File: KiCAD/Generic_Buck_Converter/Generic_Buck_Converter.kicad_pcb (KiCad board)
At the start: 4 copper layers, 17.8 x 25 mm, 20 parts, among them IC1 MAX17634C, J1 Conn_01x03

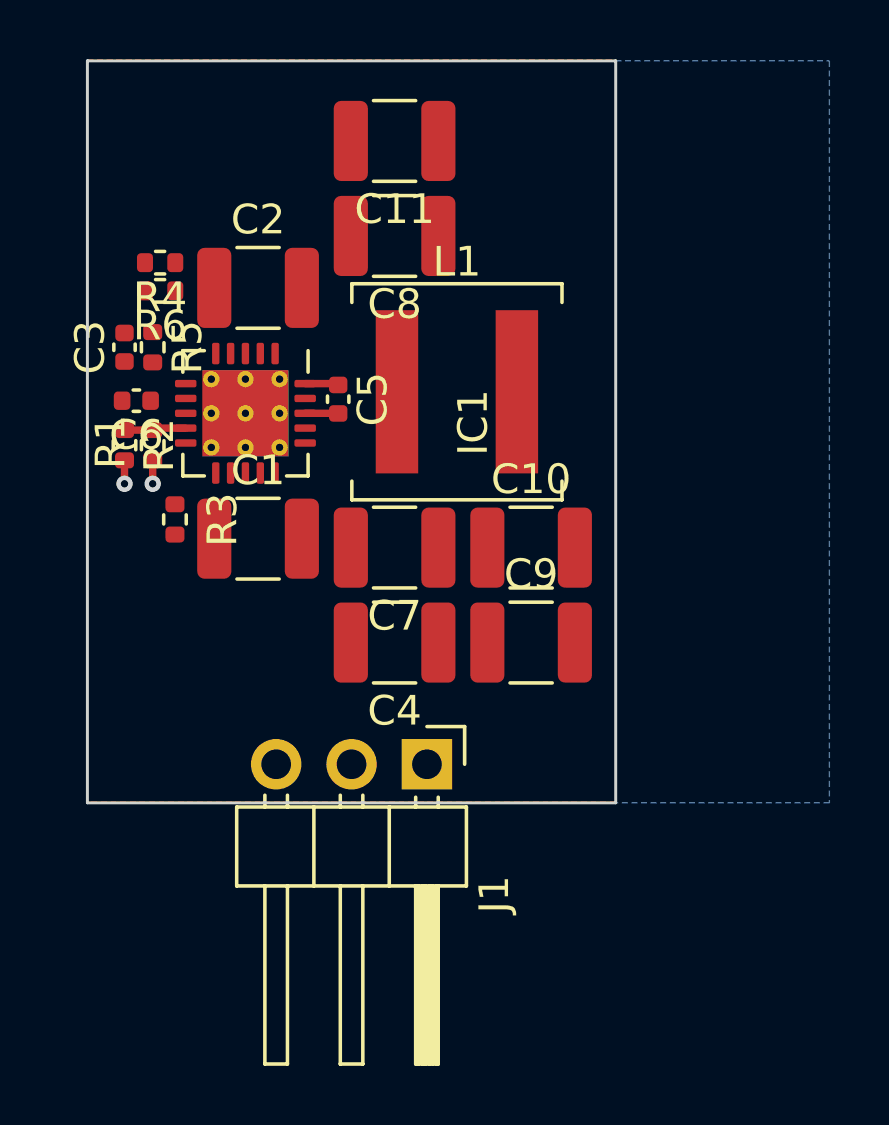
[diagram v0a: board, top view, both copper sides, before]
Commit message: Worked on main board
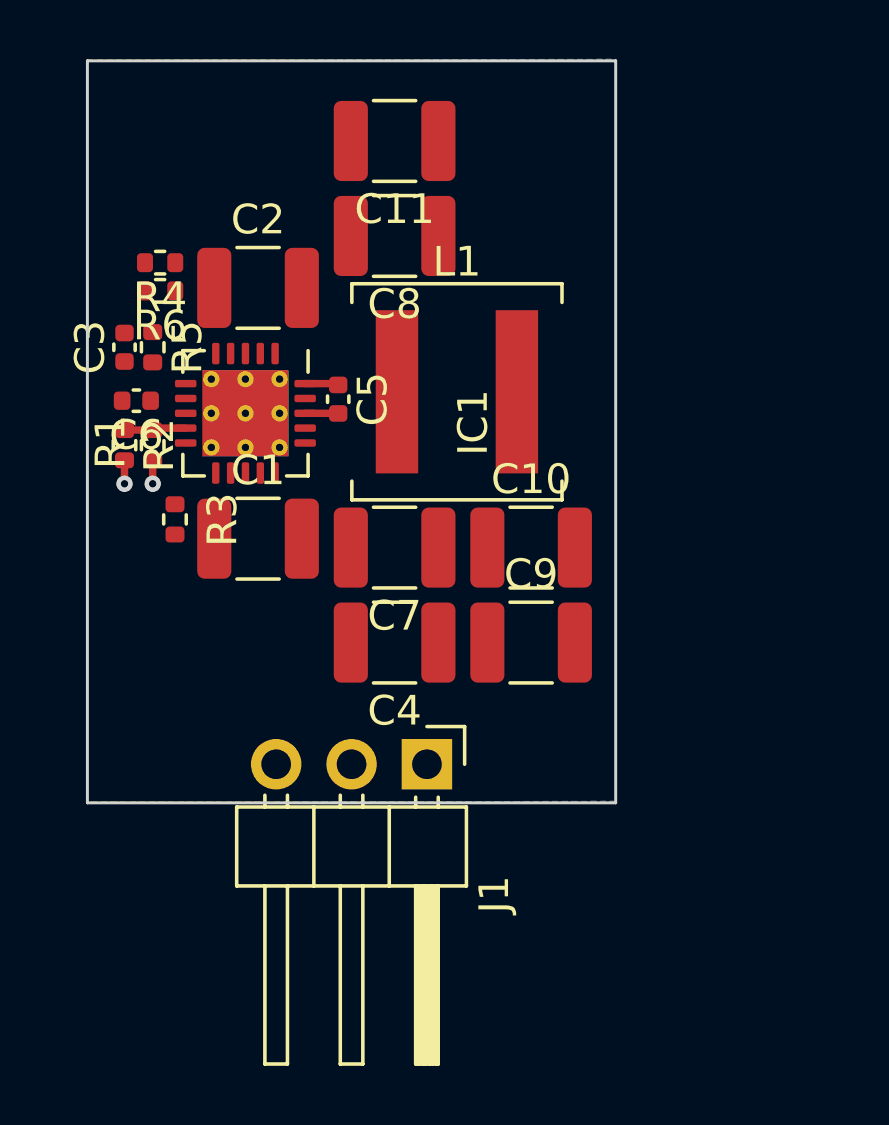
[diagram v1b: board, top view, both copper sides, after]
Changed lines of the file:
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@@
     (connect_pads (clearance 0.5))
     (min_thickness 0.25) (filled_areas_thickness no)
-    (fill yes (thermal_gap 0.5) (thermal_bridge_width 0.5))
+    (fill (thermal_gap 0.5) (thermal_bridge_width 0.5))
     (polygon
       (pts
-        (xy 125 100)
-        (xy 125 125)
+        (xy 117.8 99.95)
+        (xy 117.8 124.95)
         (xy 100 125)
         (xy 100 100)

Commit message: Buck PCB
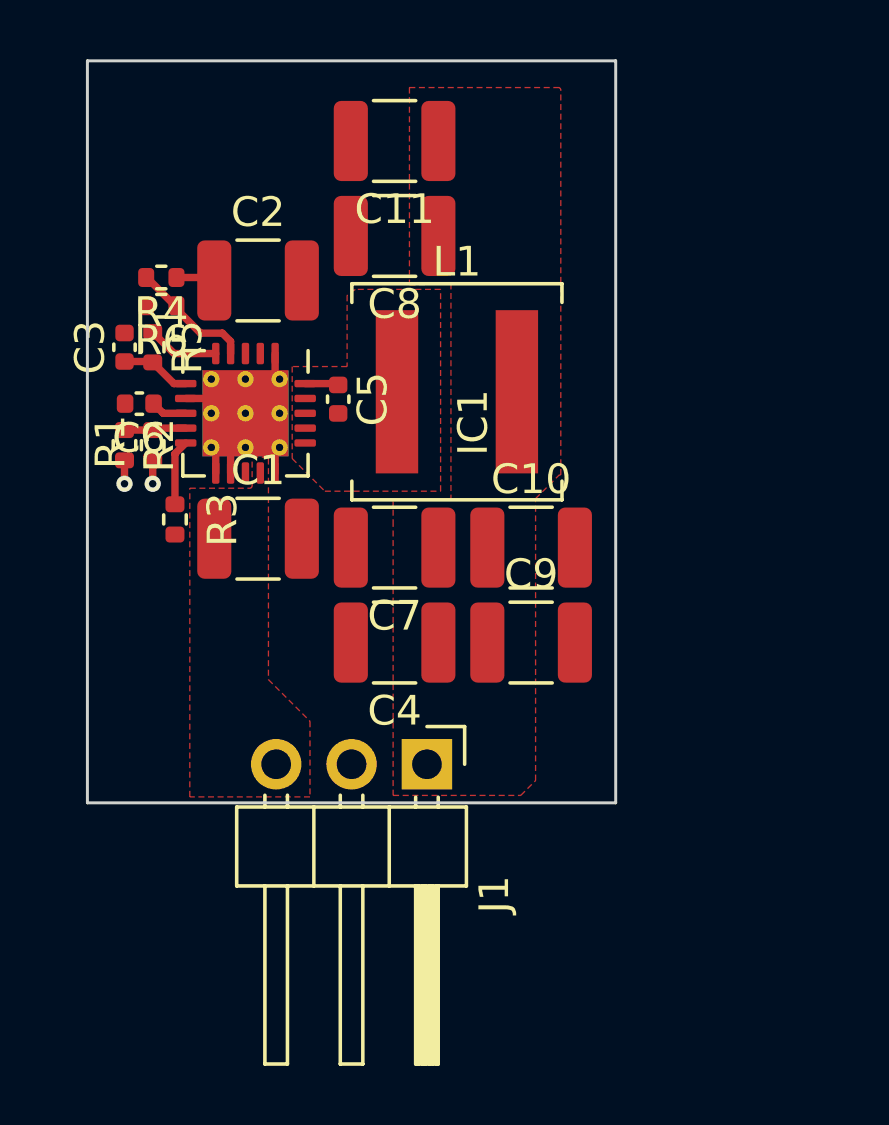
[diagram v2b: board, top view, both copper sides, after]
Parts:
- moved R4 0.50 mm to (102.5, 107.3)
- moved R6 0.50 mm to (102.5, 108.2)
- moved C2 0.25 mm to (105.8, 107.4)
- moved C6 0.14 mm to (101.8, 111.5)
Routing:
- net GND: track 0.79 -> 12.5 mm
- net Net-(IC1-EN/UVLO): track 0.00 -> 4.21 mm
- net Net-(IC1-RESET): track 0.00 -> 2.42 mm
- net Net-(IC1-INTVCC): track 0.00 -> 2.37 mm
- net Net-(IC1-RT): track 0.00 -> 2.22 mm
- net /Vin: track 0.00 -> 1.32 mm
- net Net-(IC1-SS): track 0.00 -> 1.22 mm
- net Net-(C5-Pad2): track 1.11 -> 0.01 mm
- added copper zone on F.Cu, net /Vin
- added copper zone on F.Cu, net /Vout
- added copper zone on F.Cu, net Net-(C5-Pad2)
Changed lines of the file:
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@@
   (net 13 "Net-(IC1-EN{slash}UVLO)")
   (footprint "Resistor_SMD:R_0402_1005Metric" (layer "F.Cu")
-    (at 102.45 106.8 180)
+    (at 102.49 107.3 180)
     (descr "Resistor SMD 0402 (1005 Metric), square (rectangular) end terminal, IPC_7351 nominal, (Body size source: IPC-SM-782 page 72, https://www.pcb-3d.com/wordpress/wp-content/uploads/ipc-sm-782a_amendment_1_and_2.pdf), generated with kicad-footprint-generator")
     (tags "resistor")
@@
   )
   (footprint "Resistor_SMD:R_0402_1005Metric" (layer "F.Cu")
-    (at 102.45 107.75 180)
+    (at 102.49 108.25 180)
     (descr "Resistor SMD 0402 (1005 Metric), square (rectangular) end terminal, IPC_7351 nominal, (Body size source: IPC-SM-782 page 72, https://www.pcb-3d.com/wordpress/wp-content/uploads/ipc-sm-782a_amendment_1_and_2.pdf), generated with kicad-footprint-generator")
     (tags "resistor")
@@
   )
   (footprint "Capacitor_SMD:C_1210_3225Metric" (layer "F.Cu")
-    (at 105.75 107.65)
+    (at 105.75 107.4)
     (descr "Capacitor SMD 1210 (3225 Metric), square (rectangular) end terminal, IPC_7351 nominal, (Body size source: IPC-SM-782 page 76, https://www.pcb-3d.com/wordpress/wp-content/uploads/ipc-sm-782a_amendment_1_and_2.pdf), generated with kicad-footprint-generator")
     (tags "capacitor")
@@
   )
   (footprint "Capacitor_SMD:C_0402_1005Metric" (layer "F.Cu")
-    (at 101.65 111.45 180)
+    (at 101.75 111.55 180)
     (descr "Capacitor SMD 0402 (1005 Metric), square (rectangular) end terminal, IPC_7351 nominal, (Body size source: IPC-SM-782 page 76, https://www.pcb-3d.com/wordpress/wp-content/uploads/ipc-sm-782a_amendment_1_and_2.pdf), generated with kicad-footprint-generator")
     (tags "capacitor")
@@
   (gr_rect (start 100 100) (end 117.8 125)
     (stroke (width 0.1) (type default)) (fill none) (layer "Edge.Cuts"))
+  (segment (start 103 107.3) (end 104.175 107.3) (width 0.25) (layer "F.Cu") (net 1))
+  (segment (start 104.175 107.3) (end 104.275 107.4) (width 0.25) (layer "F.Cu") (net 1))
+  (segment (start 104.325 112.875) (end 105.325 111.875) (width 0.25) (layer "F.Cu") (net 2))
   (segment (start 101.25 113.46) (end 101.25 114.25) (width 0.25) (layer "F.Cu") (net 2))
+  (segment (start 103.3125 111.375) (end 104.825 111.375) (width 0.25) (layer "F.Cu") (net 2))
+  (segment (start 104.825 113.8875) (end 104.825 112.375) (width 0.25) (layer "F.Cu") (net 2))
+  (segment (start 106.325 109.8625) (end 106.325 110.875) (width 0.25) (layer "F.Cu") (net 2))
+  (segment (start 104.825 111.375) (end 105.325 111.875) (width 0.25) (layer "F.Cu") (net 2))
+  (segment (start 106.325 110.875) (end 105.325 111.875) (width 0.25) (layer "F.Cu") (net 2))
+  (segment (start 104.825 112.375) (end 105.325 111.875) (width 0.25) (layer "F.Cu") (net 2))
+  (segment (start 106.325 112.875) (end 105.325 111.875) (width 0.25) (layer "F.Cu") (net 2))
+  (segment (start 104.325 113.8875) (end 104.325 112.875) (width 0.25) (layer "F.Cu") (net 2))
+  (segment (start 106.325 113.8875) (end 106.325 112.875) (width 0.25) (layer "F.Cu") (net 2))
   (via (at 101.25 114.25) (size 0.55) (drill 0.25) (layers "F.Cu" "B.Cu") (free) (net 2))
+  (segment (start 102.17 110.13) (end 102.2 110.16) (width 0.25) (layer "F.Cu") (net 3))
+  (segment (start 101.25 110.13) (end 102.17 110.13) (width 0.25) (layer "F.Cu") (net 3))
+  (segment (start 102.915 110.875) (end 102.2 110.16) (width 0.25) (layer "F.Cu") (net 3))
+  (segment (start 103.3125 110.875) (end 102.915 110.875) (width 0.25) (layer "F.Cu") (net 3))
   (segment (start 102.2 113.46) (end 102.2 114.25) (width 0.25) (layer "F.Cu") (net 4))
   (via (at 102.2 114.25) (size 0.55) (drill 0.25) (layers "F.Cu" "B.Cu") (free) (net 4))
@@
   (segment (start 108.405 110.875) (end 108.45 110.92) (width 0.25) (layer "F.Cu") (net 5))
   (segment (start 108.445 111.875) (end 108.45 111.88) (width 0.25) (layer "F.Cu") (net 6))
-  (segment (start 107.3375 111.875) (end 108.445 111.875) (width 0.25) (layer "F.Cu") (net 6))
+  (segment (start 102.555 111.875) (end 103.3125 111.875) (width 0.25) (layer "F.Cu") (net 7))
+  (segment (start 102.23 111.55) (end 102.555 111.875) (width 0.25) (layer "F.Cu") (net 7))
+  (segment (start 102.2 109.14) (end 102.9225 109.8625) (width 0.25) (layer "F.Cu") (net 8))
+  (segment (start 102.9225 109.8625) (end 104.325 109.8625) (width 0.25) (layer "F.Cu") (net 8))
   (segment (start 102.265 112.375) (end 103.3125 112.375) (width 0.25) (layer "F.Cu") (net 9))
   (segment (start 101.25 112.44) (end 102.2 112.44) (width 0.25) (layer "F.Cu") (net 9))
   (segment (start 102.2 112.44) (end 102.265 112.375) (width 0.25) (layer "F.Cu") (net 9))
-  (zone (net 2) (net_name "GND") (layer "F.Cu") (name "GND") (hatch edge 0.5)
-    (connect_pads (clearance 0.15))
-    (min_thickness 0.25) (filled_areas_thickness no)
+  (segment (start 102.95 113.2375) (end 103.3125 112.875) (width 0.25) (layer "F.Cu") (net 10))
+  (segment (start 102.95 114.94) (end 102.95 113.2375) (width 0.25) (layer "F.Cu") (net 10))
+  (segment (start 104.825 109.451992) (end 104.825 109.8625) (width 0.25) (layer "F.Cu") (net 13))
+  (segment (start 101.98 107.3) (end 102.000538 107.3) (width 0.25) (layer "F.Cu") (net 13))
+  (segment (start 103 108.25) (end 103 108.363173) (width 0.25) (layer "F.Cu") (net 13))
+  (segment (start 102.000538 107.3) (end 102.950538 108.25) (width 0.25) (layer "F.Cu") (net 13))
+  (segment (start 103.811827 109.175) (end 104.548008 109.175) (width 0.25) (layer "F.Cu") (net 13))
+  (segment (start 102.950538 108.25) (end 103 108.25) (width 0.25) (layer "F.Cu") (net 13))
+  (segment (start 103 108.363173) (end 103.811827 109.175) (width 0.25) (layer "F.Cu") (net 13))
+  (segment (start 104.548008 109.175) (end 104.825 109.451992) (width 0.25) (layer "F.Cu") (net 13))
+  (zone (net 1) (net_name "/Vin") (layer "F.Cu") (name "Vin") (hatch edge 0.5)
+    (priority 1)
+    (connect_pads yes (clearance 0.15))
+    (min_thickness 0.15) (filled_areas_thickness no)
     (fill yes (thermal_gap 0.5) (thermal_bridge_width 0.5))
     (polygon
       (pts
-        (xy 100 99.975)
-        (xy 117.8 99.975)
-        (xy 117.8 124.975)
-        (xy 100 124.975)
+        (xy 107.5 124.8)
+        (xy 103.45 124.8)
+        (xy 103.45 114.4)
+        (xy 105.5 114.4)
+        (xy 105.55 114.35)
+        (xy 105.55 113.35)
+        (xy 106.05 113.35)
+        (xy 106.1 113.4)
+        (xy 106.1 120.85)
+        (xy 107.5 122.25)
       )
     )
   )
-  (zone (net 2) (net_name "GND") (layers "In1.Cu" "In2.Cu") (hatch edge 0.5)
-    (connect_pads (clearance 0.5))
-    (min_thickness 0.25) (filled_areas_thickness no)
+  (zone (net 6) (net_name "Net-(C5-Pad2)") (layer "F.Cu") (name "lx") (hatch edge 0.5)
+    (priority 3)
+    (connect_pads yes (clearance 0.15))
+    (min_thickness 0.15) (filled_areas_thickness no)
+    (fill yes (thermal_gap 0.5) (thermal_bridge_width 0.5))
+    (polygon
+      (pts
+        (xy 106.9 113.4)
+        (xy 108 114.5)
+        (xy 111.9 114.5)
+        (xy 111.9 107.7)
+        (xy 111.9 107.7)
+        (xy 109.02742 107.7)
+        (xy 108.75 107.9)
+        (xy 108.75 110.3)
+        (xy 106.9 110.3)
+        (xy 106.9 113.4)
+      )
+    )
+  )
+  (zone (net 4) (net_name "/Vout") (layer "F.Cu") (name "Vout") (hatch edge 0.5)
+    (priority 1)
+    (connect_pads yes (clearance 0.15))
+    (min_thickness 0.15) (filled_areas_thickness no)
+    (fill yes (thermal_gap 0.5) (thermal_bridge_width 0.5))
+    (polygon
+      (pts
+        (xy 110.85 100.9)
+        (xy 110.85 107.553906)
+        (xy 110.85 107.553906)
+        (xy 112.920098 107.5)
+        (xy 112.25 107.5)
+        (xy 112.25 114.748684)
+        (xy 112.25 114.748684)
+        (xy 110.3 114.8)
+        (xy 110.3 115.5)
+        (xy 110.3 124.75)
+        (xy 114.6 124.75)
+        (xy 115.1 124.25)
+        (xy 115.1 114.75)
+        (xy 115.9 113.95)
+        (xy 115.95 113.95)
+        (xy 115.95 100.95)
+        (xy 115.9 100.9)
+      )
+    )
+  )
+  (zone (net 2) (net_name "GND") (layers "F.Cu" "In1.Cu" "In2.Cu" "B.Cu") (name "GND") (hatch edge 0.5)
+    (connect_pads yes (clearance 0.15))
+    (min_thickness 0.15) (filled_areas_thickness no)
     (fill yes (thermal_gap 0.5) (thermal_bridge_width 0.5))
     (polygon
       (pts
         (xy 100 100)
-        (xy 117.75 100)
-        (xy 117.75 125)
+        (xy 117.8 100)
+        (xy 117.8 125)
         (xy 100 125)
       )
     )
-  )
-  (zone (net 2) (net_name "GND") (layer "B.Cu") (hatch edge 0.5)
-    (connect_pads (clearance 0.5))
-    (min_thickness 0.25) (filled_areas_thickness no)
-    (fill (thermal_gap 0.5) (thermal_bridge_width 0.5))
-    (polygon
-      (pts
-        (xy 117.8 99.95)
-        (xy 117.8 124.95)
-        (xy 100 125)
-        (xy 100 100)
-      )
-    )
